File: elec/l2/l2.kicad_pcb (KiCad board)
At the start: 2 copper layers, 170.8 x 168.4 mm, 34 parts, among them J1 Conn_01x06, J2 Conn_01x06, J3 Conn_01x04, J5 Conn_01x08, SW101 SW_Push, U2 DEV-15583

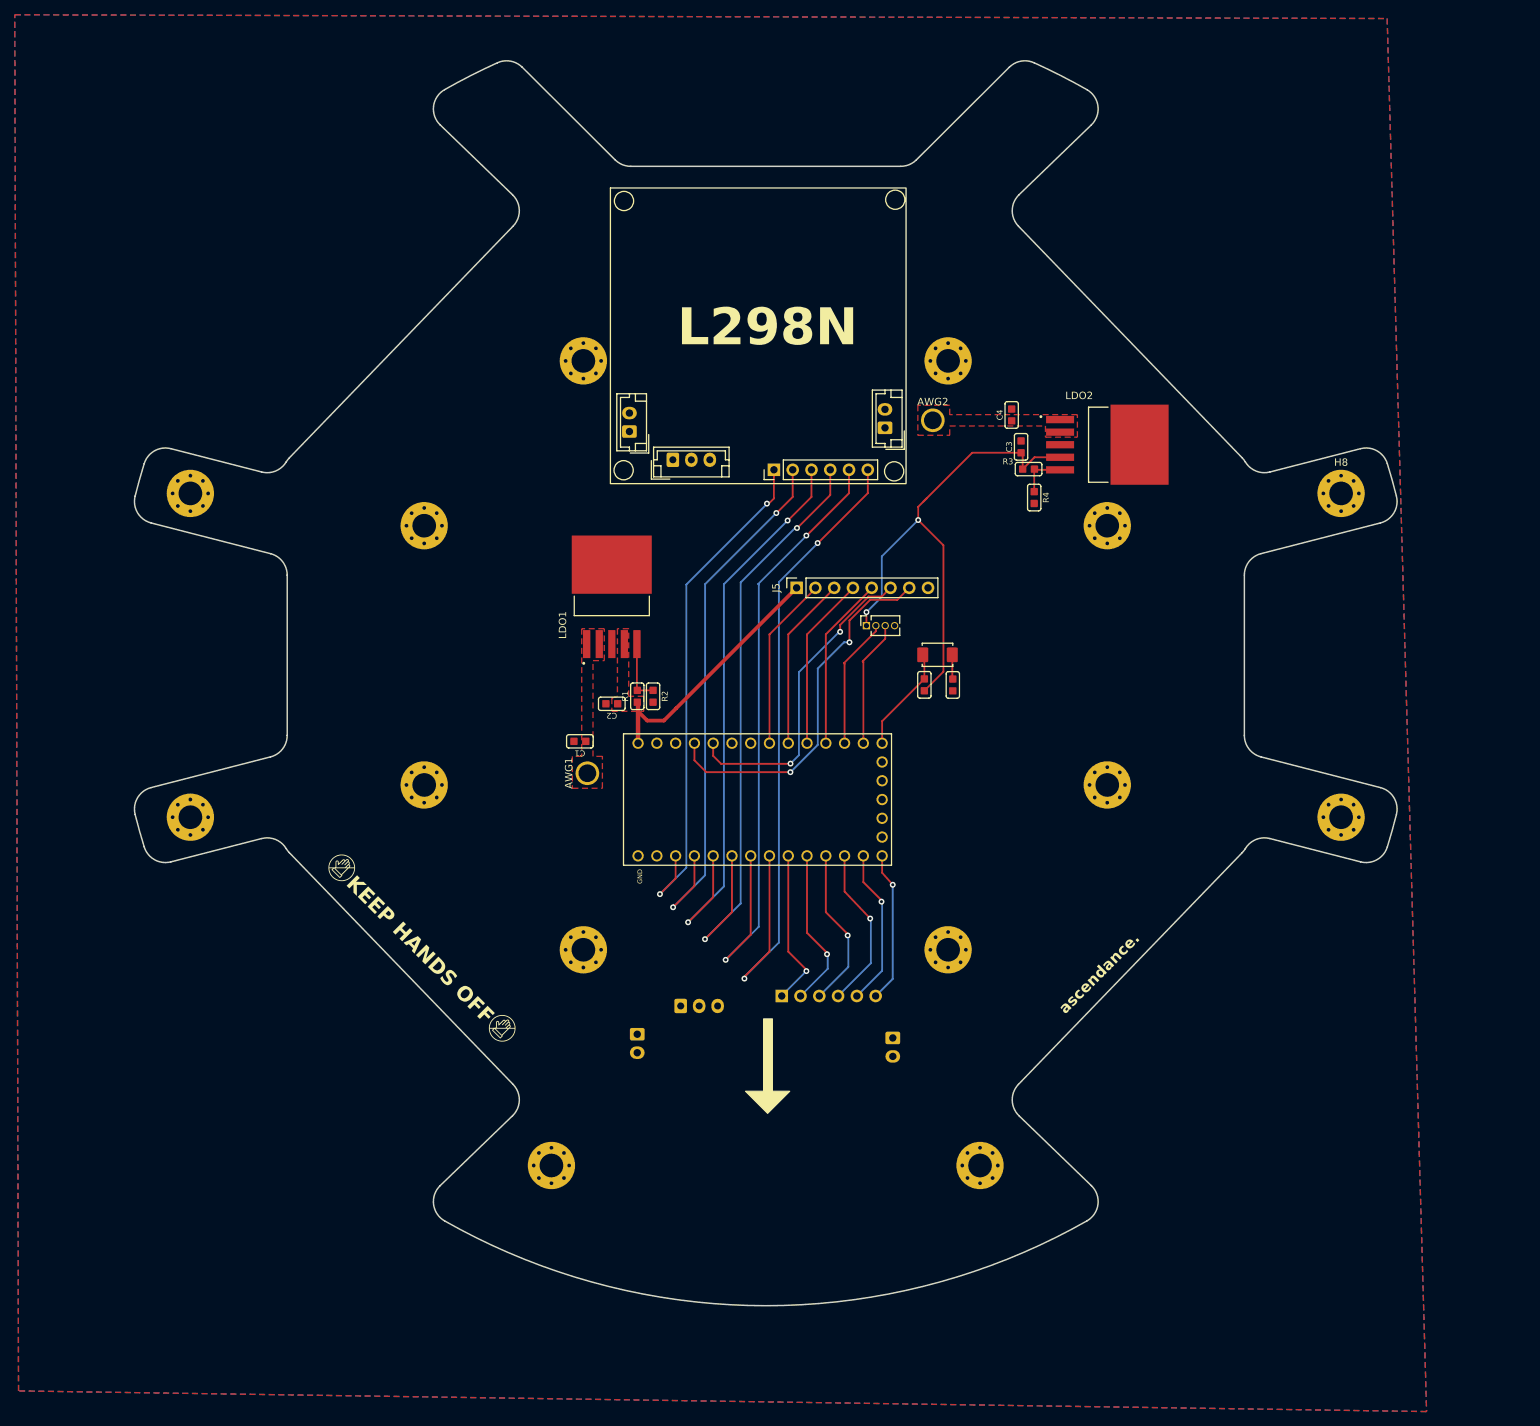
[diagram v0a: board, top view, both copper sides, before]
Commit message: 2024-02-28 production
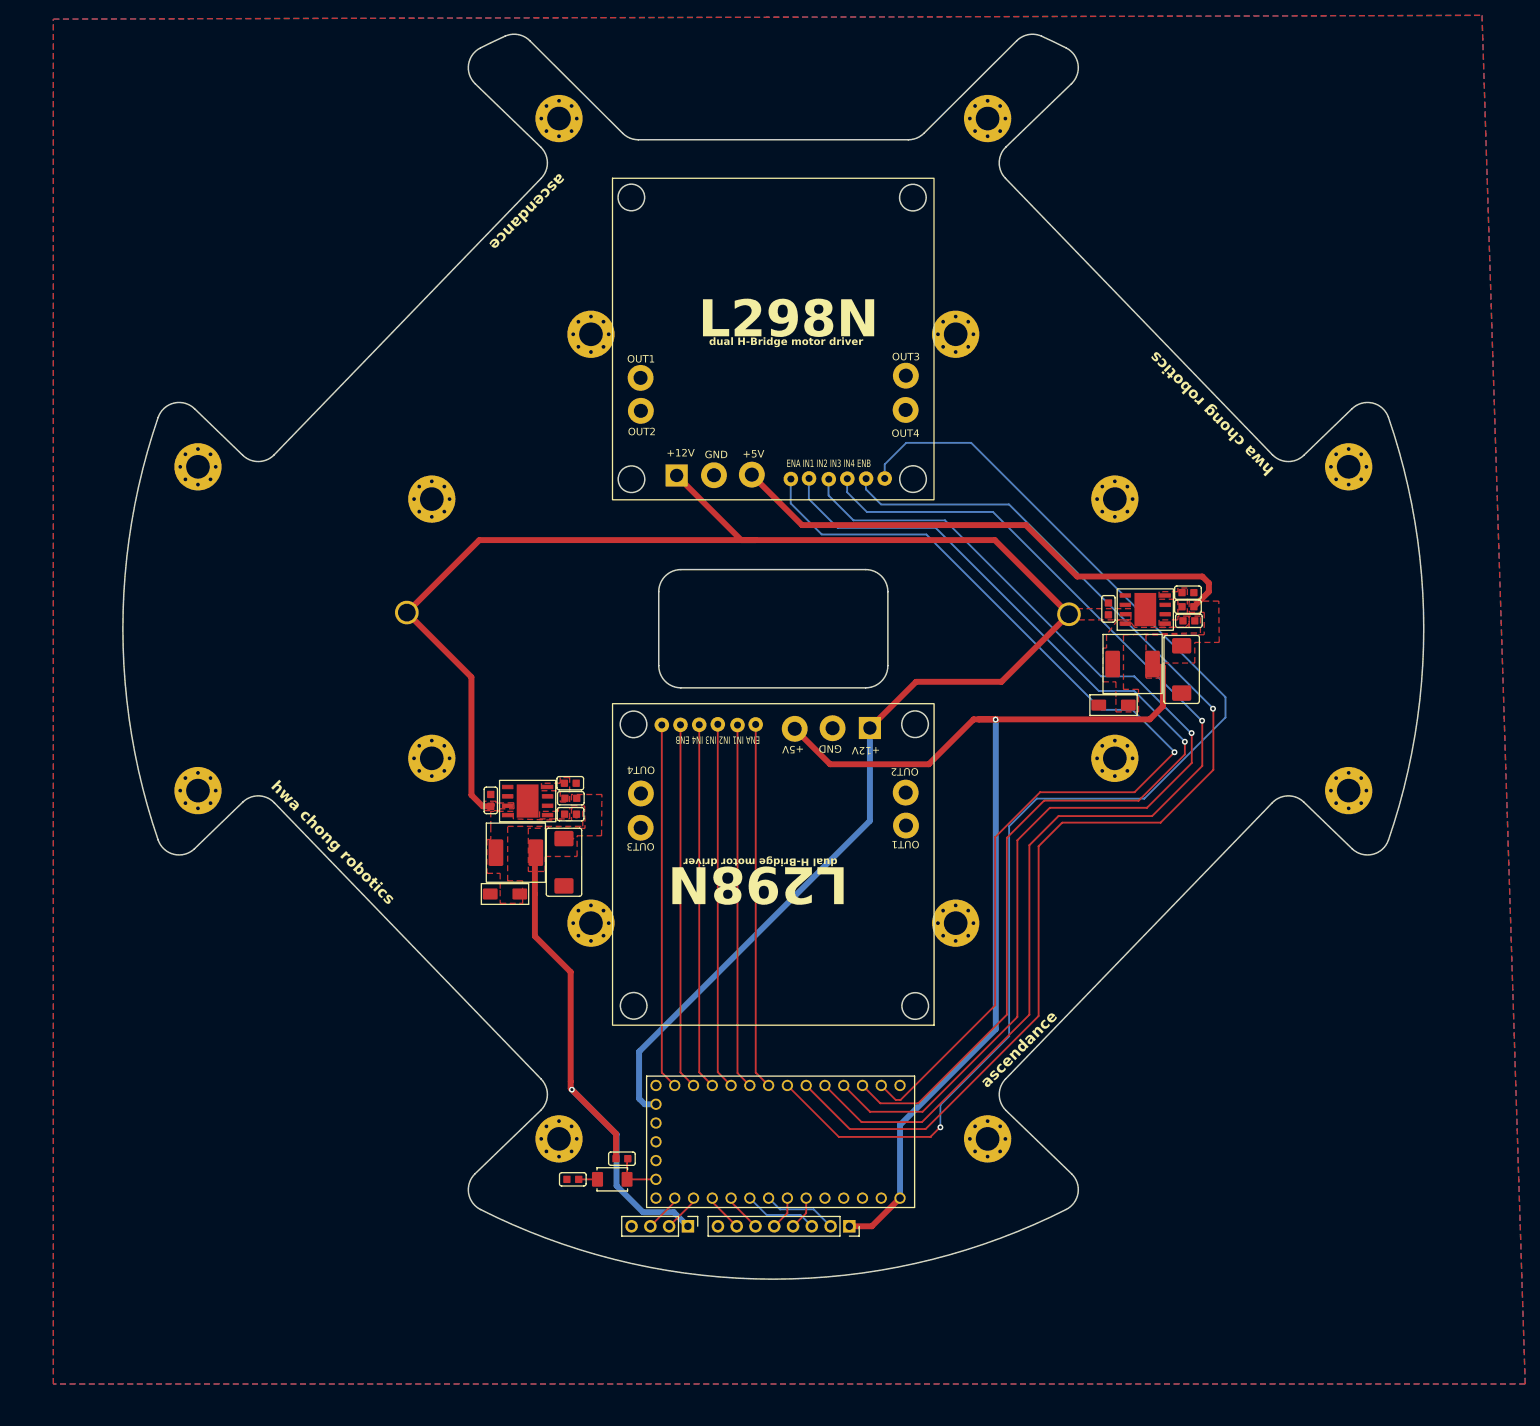
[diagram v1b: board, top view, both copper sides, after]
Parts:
- removed AWG1, AWG2: MountingHole, l2:14 AWG
- removed LDO1, LDO2: ~, TLF1963:TLF1963TBATMA1 footprint
- added C5: 220u, l2:EIA-7343-D, F.Cu at (86.2, 126.3)
- added C6: C, l2:cap0603, F.Cu at (76.3, 118.0)
- added D1: B340, hy:DIOM5025X220N, F.Cu at (160.6, 105.1)
- added D2: B340, hy:DIOM5025X220N, F.Cu at (78.3, 130.6)
- added H1: MountingHole_Pad, MountingHole:MountingHole_3.2mm_M3_Pad_Via, F.Cu at (85.6, 25.7)
- added H2: MountingHole_Pad, MountingHole:MountingHole_3.2mm_M3_Pad_Via, F.Cu at (143.6, 25.7)
- added L1: 15uH, l2:0630 One Piece Inductor, F.Cu at (163.2, 99.5)
- added L2: 15uH, l2:0630 One Piece Inductor, F.Cu at (79.7, 125.0)
- added U1: TPS5430DDA, l2:TI_SO-PowerPAD-8, F.Cu at (164.9, 92.2)
- added U3: TPS5430DDA, l2:TI_SO-PowerPAD-8, F.Cu at (81.3, 118.1)
- added batawg1: +12V, l2:14 AWG, F.Cu at (154.6, 92.8)
- added batawg2: +12V, l2:14 AWG, F.Cu at (65.0, 92.6)
- C1: value 10u -> 10n
- C2: value 10u -> 220u; footprint l2:cap0603 -> l2:EIA-7343-D
- C3: value 10u -> C
- J1: value Conn_01x06 -> Conn_01x13; moved to F.Cu
- J2: value Conn_01x06 -> Conn_01x13
- J3: footprint Connector_PinSocket_1.27mm:PinSocket_1x04_P1.27mm_Vertical -> Connector_PinHeader_2.54mm:PinHeader_1x04_P2.54mm_Vertical
- moved H7 123.3 mm to (36.7, 72.8)
- moved H11 123.0 mm to (36.7, 116.6)
- moved J1 110.2 mm to (114.6, 52.3)
- moved H10 93.5 mm to (160.8, 112.3)
- moved H6 93.5 mm to (160.8, 77.2)
- moved J5 86.7 mm to (124.9, 175.6), turned to -90 degrees
- moved J3 84.8 mm to (103.0, 175.6), turned to -90 degrees
- moved R102 84.4 mm to (87.4, 169.2), turned to 180 degrees
- moved C1 84.0 mm to (170.8, 93.7), turned to 0 degrees
- moved SW101 83.5 mm to (92.8, 169.2), turned to 0 degrees
- moved C4 80.5 mm to (87.1, 119.8), turned to 180 degrees
- moved C2 77.2 mm to (169.8, 100.3), turned to -90 degrees
- moved R3 76.3 mm to (87.2, 117.7), turned to 180 degrees
- moved R101 76.1 mm to (94.1, 166.4), turned to 0 degrees
- moved R1 75.5 mm to (170.7, 91.8), turned to 180 degrees
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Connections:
- C1 pad 1: +12V -> Net-(U1-BOOT)
- C1 pad 2: GND -> Net-(D1-K)
- C3 pad 1: +3V3 -> +12V
- C4 pad 1: +12V -> Net-(D2-K)
- C4 pad 2: GND -> Net-(U3-BOOT)
- J1 pad 1: /ENA -> unconnected-(J1-Pin_1-Pad1)
- J1 pad 2: /ENB -> unconnected-(J1-Pin_2-Pad2)
- J1 pad 3: /IN1 -> +12V
- J1 pad 4: /IN2 -> GND
- J1 pad 5: /IN3 -> +5V
- J1 pad 6: /IN4 -> /1-ENA
- J2 pad 1: /ENA -> unconnected-(J2-Pin_1-Pad1)
- J2 pad 2: /ENB -> unconnected-(J2-Pin_2-Pad2)
- J2 pad 3: /IN1 -> +12V
- J2 pad 4: /IN2 -> GND
- J2 pad 5: /IN3 -> +5V
- J2 pad 6: /IN4 -> /2-ENA
- U2 pad 0: unconnected-(U2-Pad0) -> /1-ENA
- U2 pad 1: /ENA -> /1-IN1
- U2 pad 10: /IN2 -> /2-IN4
- U2 pad 11: /IN3 -> /2-ENB
- U2 pad 12: /IN4 -> unconnected-(U2-Pad12)
- U2 pad 13: /RESET -> unconnected-(U2-Pad13)
- U2 pad 16: /C TX -> /COM SDA
- U2 pad 17: /C RX -> /COM SDL
- U2 pad 2: /ENB -> /1-IN2
- U2 pad 20: unconnected-(U2-Pad20) -> /C TX
- U2 pad 21: unconnected-(U2-Pad21) -> /C RX
- U2 pad 22: /COM SDL -> unconnected-(U2-Pad22)
- U2 pad 23: /COM SDA -> unconnected-(U2-Pad23)
- U2 pad 3: /IN1 -> /1-IN3
- U2 pad 4: /IN2 -> /1-IN4
- U2 pad 5: /IN3 -> /1-ENB
- U2 pad 6: /IN4 -> /2-ENA
- U2 pad 7: /ENA -> /2-IN1
- U2 pad 8: /ENB -> /2-IN2
- U2 pad 9: /IN1 -> /2-IN3
- U2 pad ON-OFF: unconnected-(U2-ON/OFF-PadON-OFF) -> /RESET
- U2 pad VBAT: unconnected-(U2-PadVBAT) -> +12V
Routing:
- net +12V: track 0.00 -> 243.4 mm
- net +5V: track 36.1 -> 215.0 mm, vias 0 -> 1
- net /1-ENB: track 0.00 -> 170.4 mm, vias 0 -> 1
- net /1-IN4: track 0.00 -> 160.1 mm, vias 0 -> 1
- net /1-IN3: track 0.00 -> 155.3 mm, vias 0 -> 1
- net /1-IN2: track 0.00 -> 150.9 mm, vias 0 -> 1
- net /1-IN1: track 0.00 -> 147.2 mm, vias 0 -> 1
- net /1-ENA: track 0.00 -> 142.5 mm, vias 0 -> 1
- net /IN4: track 114.4 -> 0.00 mm, vias 3 -> 0
- net /IN3: track 110.7 -> 0.00 mm, vias 3 -> 0
- net /IN2: track 106.0 -> 0.00 mm, vias 3 -> 0
- net /IN1: track 100.9 -> 0.00 mm, vias 3 -> 0
- net /ENB: track 96.1 -> 0.00 mm, vias 3 -> 0
- net /ENA: track 92.8 -> 0.00 mm, vias 3 -> 0
- net /2-IN4: track 0.00 -> 49.7 mm
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- added copper zone on F.Cu, net +3V3
- added copper zone on B.Cu, net GND
- added copper zone on F.Cu, net GND
- added copper zone on F.Cu, net Net-(D1-K)
- added copper zone on F.Cu, net Net-(D2-K)
- added copper zone on F.Cu, net Net-(U1-BOOT)
- added copper zone on F.Cu, net Net-(U1-VSENSE)
- added copper zone on F.Cu, net Net-(U3-BOOT)
- added copper zone on F.Cu, net Net-(U3-VSENSE)
- removed copper zone on B.Cu, net (none)
- removed copper zone on F.Cu, net (none)
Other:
- board size 170.8 x 168.4 mm -> 176 x 168.4 mm
- board text added: "ascendance"
- board text removed: "KEEP HANDS OFF"
- board text removed: "ascendance."
